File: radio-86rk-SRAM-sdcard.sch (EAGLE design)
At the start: 15 parts, among them IC1 LM1117 3.3V, U1 ATMEGA328P, U2 HEF4050B

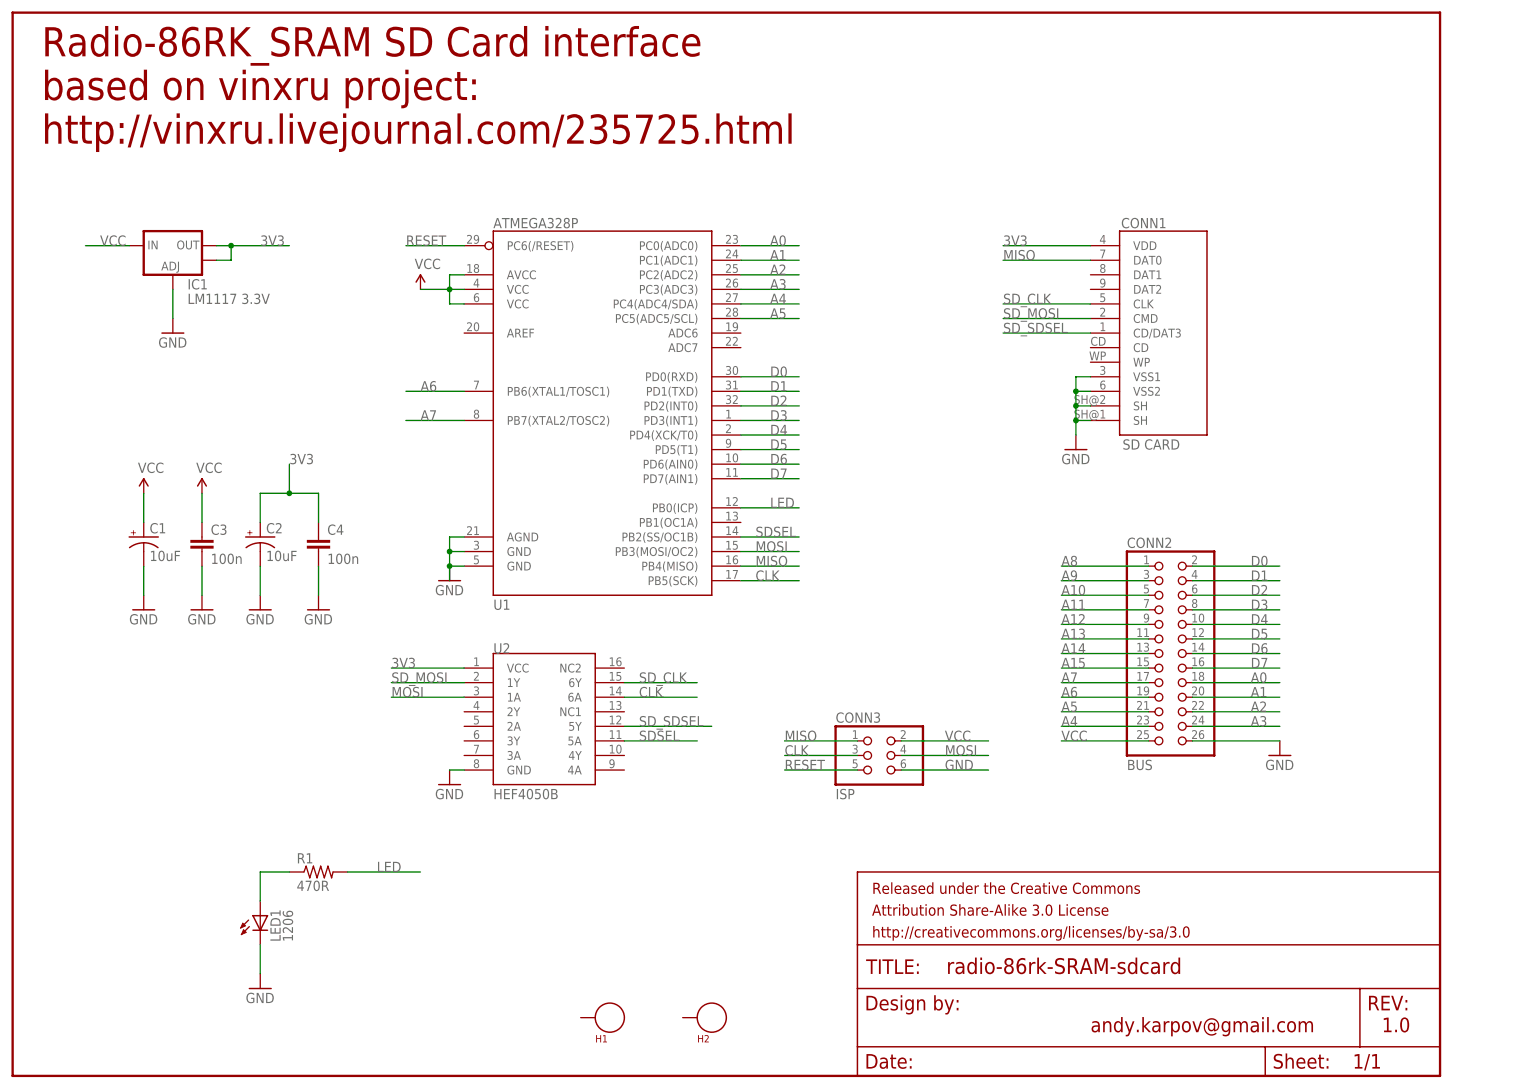
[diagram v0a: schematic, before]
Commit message: Recovered v2.0 of the PCB
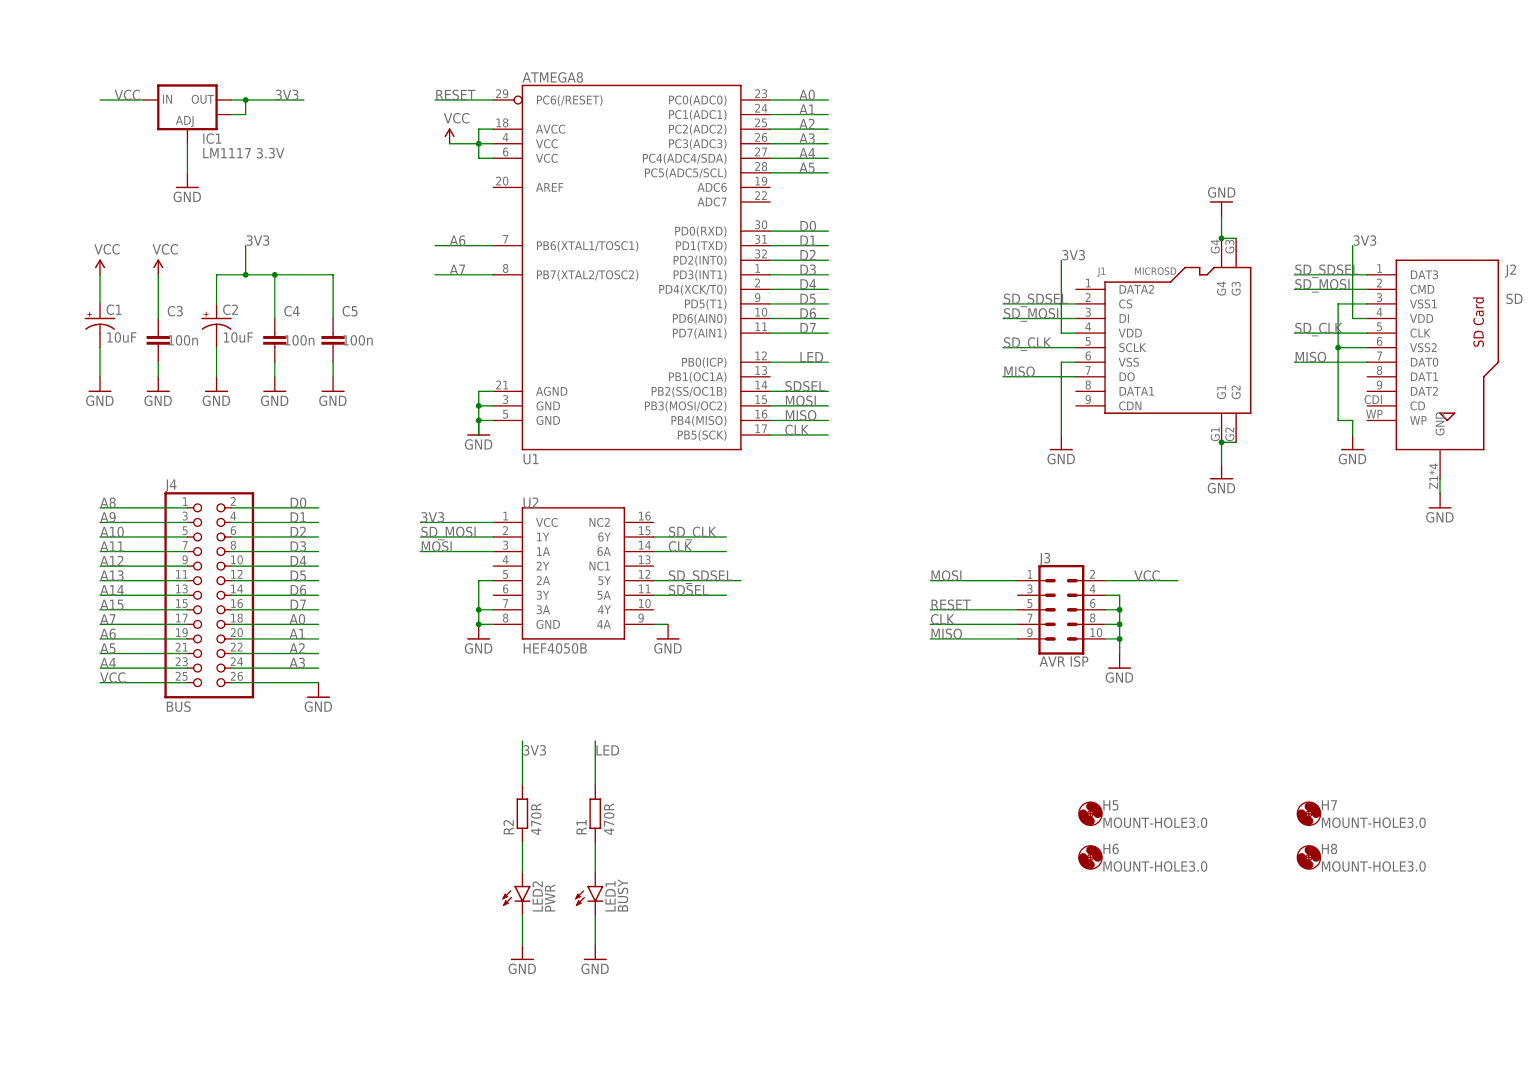
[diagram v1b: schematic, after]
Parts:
- removed CONN1: SD CARD, SparkFun-Connectors:SD_CARD_SOCKET4UCON
- removed CONN2: BUS, 2x13header:PINHD-2X13
- removed CONN3: ISP, SparkFun-Connectors:PINHD-2X3
- removed FRAME1: FRAME-LETTER, SparkFun-Aesthetics:FRAME-LETTER
- removed H1, H2: SEW_HOLE, LilyPad-Wearables:SEW_HOLE
- added C5: 100n, rcl:C-EUC0805
- added H5, H6, H7, H8: MOUNT-HOLE3.0, holes:MOUNT-HOLE3.0
- added J1: MICROSD, OPL_Connector:MICRO-SD-CARD-HOLDER-9P
- added J2: SD, Wurth_Elektronik_Electromechanic_Input-Output_Connectors_rev18b:693063010911
- added J3: AVR ISP, SparkFun-Connectors:CONN_05X2SHD_LOCK
- added J4: BUS, 2x13header:PINHD-2X13
- added LED2: PWR, led:LEDCHIP-LED0805
- added R2: 470R, rcl:R-EU_R0805
- C3, C4: device SparkFun-Capacitors:CAP1206 -> rcl:C-EUC0805
- LED1: value 1206 -> BUSY; device adafruit:LEDCHIPLED_1206 -> led:LEDCHIP-LED0805
- R1: device SparkFun-Passives:RESISTOR1206 -> rcl:R-EU_R0805
- U1: value ATMEGA328P -> ATMEGA8
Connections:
- new net N$2: LED2.A, R2.1
- net 3V3: now also C5.1, J1.VDD, J2.VDD, R2.2; no longer CONN1.VDD
- net A0: now also J4.18; no longer CONN2.18
- net A1: now also J4.20; no longer CONN2.20
- net A10: now also J4.5; no longer CONN2.5
- net A11: now also J4.7; no longer CONN2.7
- net A12: now also J4.9; no longer CONN2.9
- net A13: now also J4.11; no longer CONN2.11
- net A14: now also J4.13; no longer CONN2.13
- net A15: now also J4.15; no longer CONN2.15
- net A2: now also J4.22; no longer CONN2.22
- net A3: now also J4.24; no longer CONN2.24
- net A4: now also J4.23; no longer CONN2.23
- net A5: now also J4.21; no longer CONN2.21
- net A6: now also J4.19; no longer CONN2.19
- net A7: now also J4.17; no longer CONN2.17
- net A8: now also J4.1; no longer CONN2.1
- net A9: now also J4.3; no longer CONN2.3
- net CLK: now also J3.7; no longer CONN3.3
- net D0: now also J4.2; no longer CONN2.2
- net D1: now also J4.4; no longer CONN2.4
- net D2: now also J4.6; no longer CONN2.6
- net D3: now also J4.8; no longer CONN2.8
- net D4: now also J4.10; no longer CONN2.10
- net D5: now also J4.12; no longer CONN2.12
- net D6: now also J4.14; no longer CONN2.14
- net D7: now also J4.16; no longer CONN2.16
- net GND: now also C5.2, J1.G1, J1.G2, J1.G3, J1.G4, J1.VSS, J2.GND, J2.VSS1, J2.VSS2, J3.10, J3.4, J3.6, J3.8, J4.26, LED2.C, U2.2A, U2.3A, U2.4A; no longer CONN1.SH@1, CONN1.SH@2, CONN1.VSS1, CONN1.VSS2, CONN2.26, CONN3.6
- net MISO: now also J1.DO, J2.DAT0, J3.9; no longer CONN1.DAT0, CONN3.1
- net MOSI: now also J3.1; no longer CONN3.4
- net RESET: now also J3.5; no longer CONN3.5
- net SD_CLK: now also J1.SCLK, J2.CLK; no longer CONN1.CLK
- net SD_MOSI: now also J1.DI, J2.CMD; no longer CONN1.CMD
- net SD_SDSEL: now also J1.CS, J2.DAT3; no longer CONN1.CD/DAT3
- net VCC: now also J3.2, J4.25; no longer CONN2.25, CONN3.2
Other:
- note removed: "1.0"
- note removed: "Radio-86RK_SRAM SD Card interface based on vinxru project: http://vinxru.livejournal.com/235725.html"
- note removed: "andy.karpov@gmail.com"
- moved on the sheet: C1, C2, C3, C4, IC1, U1, U2
